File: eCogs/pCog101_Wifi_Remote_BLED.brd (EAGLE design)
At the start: 47.5 x 28 mm, 45 parts

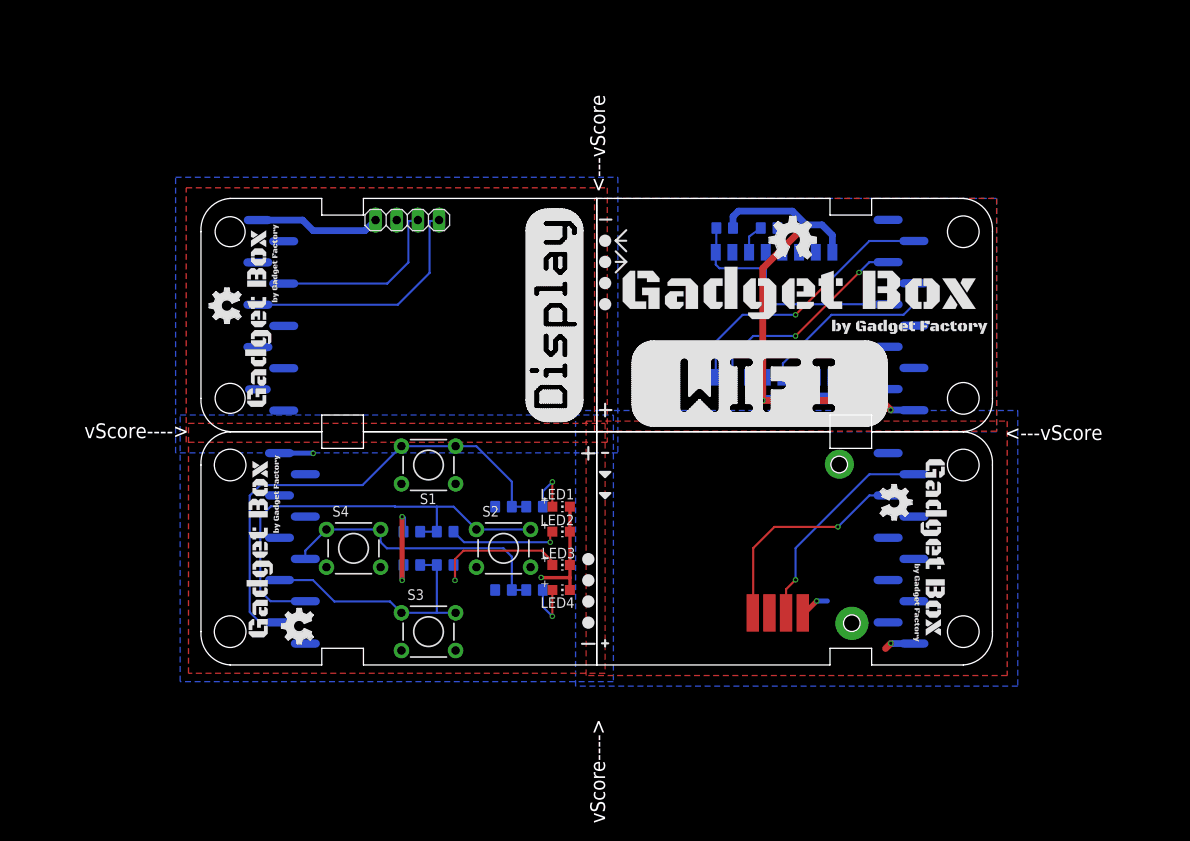
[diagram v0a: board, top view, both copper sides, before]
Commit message: Reorganized
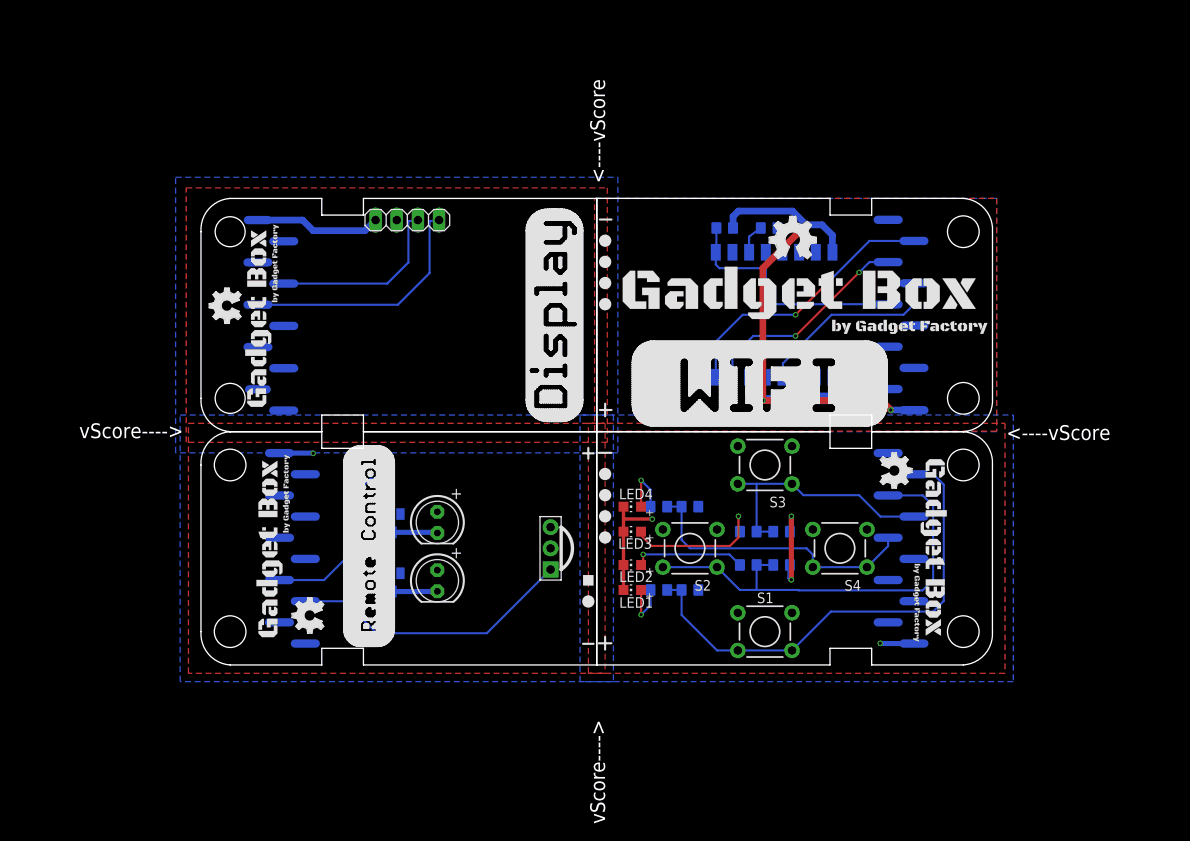
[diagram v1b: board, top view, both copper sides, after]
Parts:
- removed U$19: (no value), ohw-logo:OSHW_FILLX200_NOTEXT
- added IR1, IR2: (no value), adafruit:LED5MM
- added R13: 10K, GadgetFactory:0805
- added T1, T3: MMBT3904LT1G, transistor:SOT23-BEC
- added U1: PNA460XM, adafruit:PNA460XM
- R1: value 390 -> 1.0 K; device GadgetFactory:0805 -> rcl-ez:R0805
- R2, R4, R6, R8: value 10K -> 390
- R3, R5, R7: value 390 -> 10K
- U$10, U$12: device GadgetFactory:GADGETBOX_SMALL -> ohw-logo:OSHW_FILLX150_NOTEXT
- U$11: device ohw-logo:OSHW_FILLX150_NOTEXT -> GadgetFactory:GADGETBOX_SMALL
- U$13: device ohw-logo:OSHW_FILLX150_NOTEXT -> GadgetFactory:GADGETBOX_TEXT
- U$14: device GadgetFactory:GADGETBOX_TEXT -> eCogs:LEGEND_DIO
- U$18: device eCogs:LEGEND_DIO -> ohw-logo:OSHW_FILLX200_NOTEXT
- U$2: device eCogs:LEGEND_DIO -> eCogs:LEGEND_PWM
- U$7: value JOYSTICK-PSP1000 -> (none); device SparkFun:JOYSTICK-PSP1000 -> eCogs:LEGEND_DIO
- U$8: device eCogs:LEGEND_ANALOG -> eCogs:LEGEND_DIO
- U$9: device eCogs:LEGEND_ANALOG -> GadgetFactory:GADGETBOX_SMALL
- moved U$11 77.2 mm to (7.45, 41.6), turned to 90 degrees
- moved U$13 67.2 mm to (72.4, 44.4), turned to 0 degrees
- moved S4 58.4 mm to (77.2, 14.0), turned to 180 degrees
- moved S3 45.1 mm to (68.2, 24.0), turned to 180 degrees
- moved S1 45.1 mm to (68.2, 4.00), turned to 180 degrees
- moved R6 40.6 mm to (66.2, 16.0), turned to 0 degrees
- moved R4 40.6 mm to (66.2, 12.0), turned to 0 degrees
- moved R5 40.4 mm to (70.2, 12.0), turned to 0 degrees
- moved U$9 39.9 mm to (88.4, 14.0), turned to 270 degrees
- moved R7 30.5 mm to (70.2, 16.0), turned to 0 degrees
- moved R3 30.2 mm to (59.2, 9.00), turned to 0 degrees
- moved R11 24.1 mm to (76.2, 32.0), turned to 0 degrees
- moved U$14 23.4 mm to (49.0, 43.3), turned to 180 degrees
- moved S2 22.4 mm to (59.2, 14.0), turned to 180 degrees
- moved U$7 21.7 mm to (49.0, 20.4)
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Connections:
- removed net HORIZONTAL: ECOG1.G1, U$7.X
- removed net VERTICAL: ECOG1.G0, U$7.Y
- new net BLAST_RX: ECOG.G0
- new net BLAST_TX: ECOG.G3
- new net N$12: R13.1, X1.3
- new net N$7: IR1.K, T1.C
- new net N$8: R10.1, X1.11
- new net RECEIVE: ECOG.G1, U1.1
- new net TRANSMIT: ECOG.G2, R1.1
- net 1: now also ECOG1.G0, R2.1, R3.2; no longer ECOG.G0, R1.1, R2.2
- net 2: now also ECOG1.G1, R4.1, R5.2; no longer ECOG.G1, R3.1, R4.2
- net 3: now also ECOG1.G2, R6.1, R7.2; no longer ECOG.G2, R5.1, R6.2
- net 3V3: now also IR1.A, IR2.A, R10.2, R13.2, U1.3; no longer R11.2, R9.2, U$7.VCC
- net 4: now also ECOG1.G3, R8.1, R9.2; no longer ECOG.G3, R7.1, R8.2
- net GND: now also R11.1, R3.1, R5.1, R7.1, R9.1, T1.E, T3.E, U1.2; no longer R10.1, R2.1, R4.1, R6.1, R8.1, U$7.GND
- net N$1: now also R2.2; no longer R1.2
- net N$10: now also R1.2, T1.B, T3.B; no longer R10.2, X1.10
- net N$11: now also R11.2, X1.10; no longer R12.1, X1.3
- net N$2: now also R4.2; no longer R3.2
- net N$3: now also R6.2; no longer R5.2
- net N$4: now also R8.2; no longer R7.2
- net N$9: now also IR2.K, T3.C; no longer R9.1, X1.11
- net RESET: now also R12.1; no longer R11.1
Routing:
- net RECEIVE: track 0.00 -> 34.2 mm
- net HORIZONTAL: track 26.6 -> 0.00 mm, vias 1 -> 0
- net VERTICAL: track 26.1 -> 0.00 mm, vias 1 -> 0
- net TRANSMIT: track 0.00 -> 21.6 mm
- net N$10: track 2.90 -> 9.72 mm
- net N$7: track 0.00 -> 5.39 mm
- net N$12: track 0.00 -> 3.63 mm
- net GND: track 28.4 -> 24.8 mm, vias 4 -> 3
- net N$9: track 2.56 -> 5.41 mm
- net N$8: track 0.00 -> 2.56 mm
- net N$11: track 3.63 -> 2.90 mm
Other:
- board text added: "+"
- board text added: "<----vScore"
- board text added: "RECEIVE"
- board text added: "Remote Control"
- board text added: "TRANSMIT"
- board text added: "XC0"
- board text added: "XC1"
- board text added: "XC2"
- board text added: "XC3"
- board text added: "ecog107 v2.0"
- board text added: "ecog107.GadgetFactory.net"
- board text removed: "0"
- board text removed: "1"
- board text removed: "2"
- board text removed: "3"
- board text removed: "<---vScore"
- board text removed: "Horizontal"
- board text removed: "PSP Thumb Joystick"
- board text removed: "Vert"
- board text removed: "ecog104 v2.0"
- board text removed: "ecog104.GadgetFactory.net"
